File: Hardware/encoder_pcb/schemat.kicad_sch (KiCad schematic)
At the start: 8 parts, among them IC1 AS5040

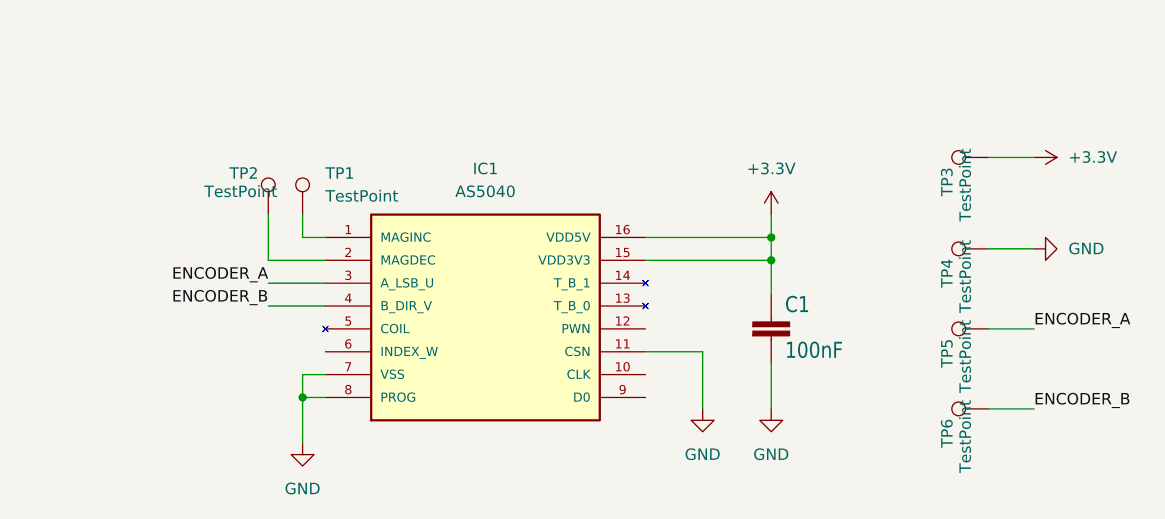
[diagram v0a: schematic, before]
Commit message: Minor fixes in schematics, added gerbers and schematics pdfs
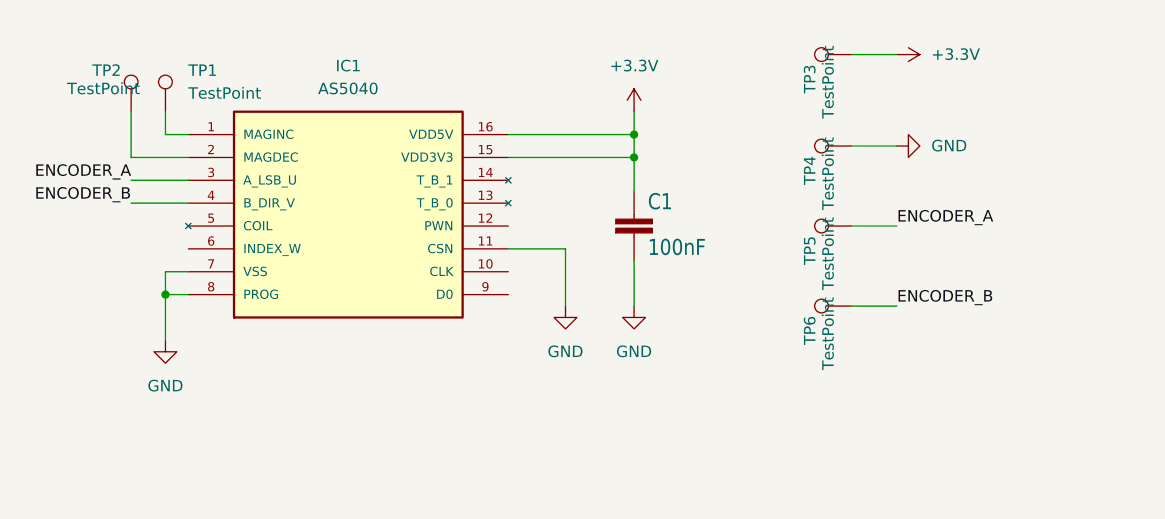
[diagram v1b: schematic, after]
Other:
- moved on the sheet: C1, IC1, TP1, TP2, TP3, TP4, TP5, TP6
